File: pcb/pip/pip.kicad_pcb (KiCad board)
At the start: 2 copper layers, 41.9 x 23.9 mm, 30 parts, among them J1 USBPCB, Q1 BC847, SW1 FLASH, SW2 RESET, SW3 BUTTON_A, SW4 BUTTON_B, U1 74HC595, U2 W25Q32JVSS, U3 CH552G

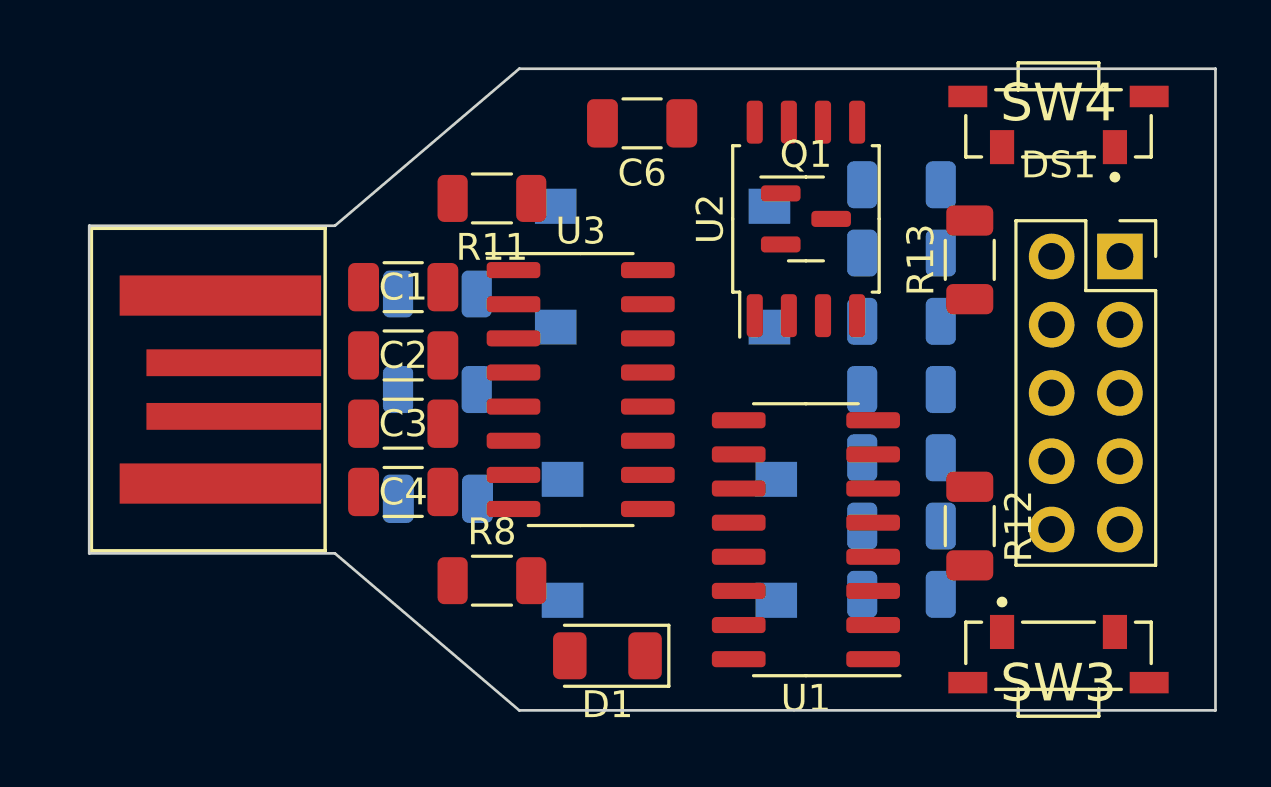
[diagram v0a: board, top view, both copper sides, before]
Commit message: pcb design
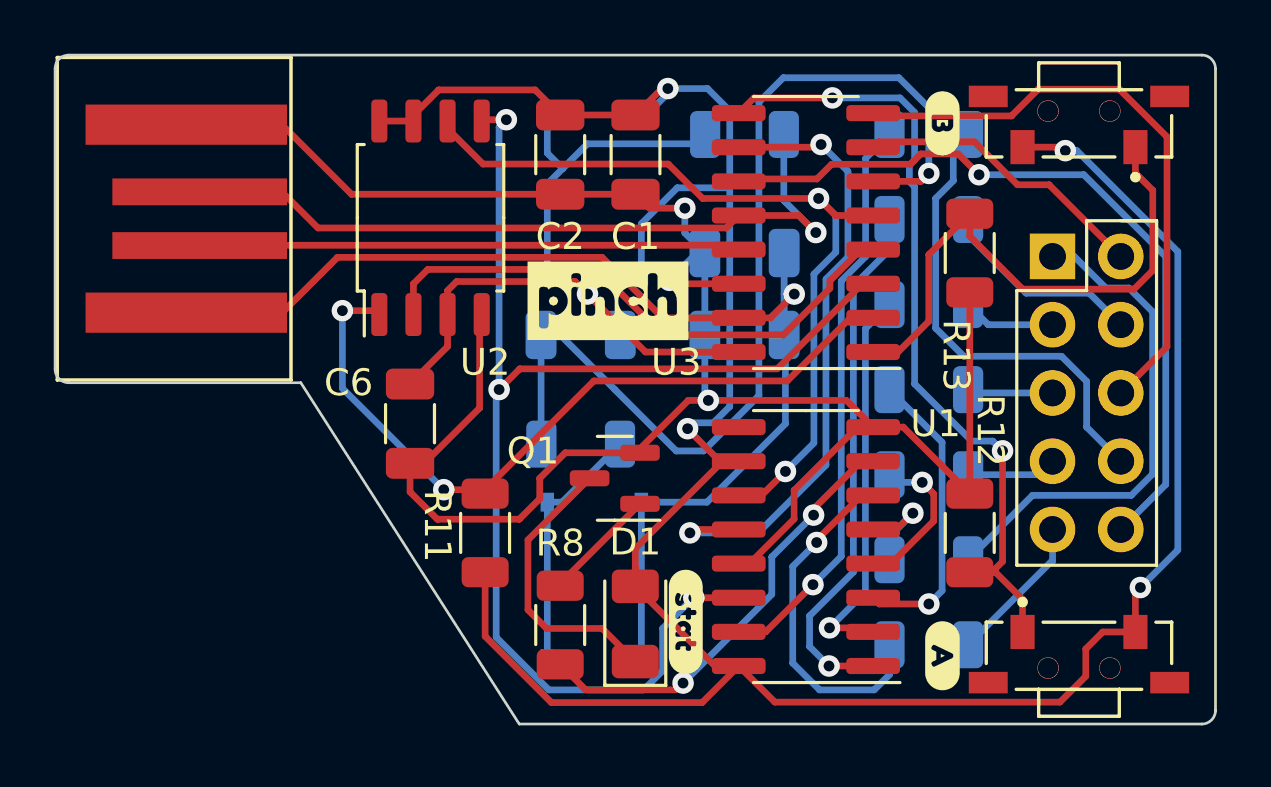
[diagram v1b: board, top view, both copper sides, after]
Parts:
- added kibuzzard-63727E71: G***, kibuzzard-63727E71, F.Cu at (149.9, 101.3)
- added kibuzzard-63727E80: G***, kibuzzard-63727E80, F.Cu at (149.9, 81.5)
- added kibuzzard-637287DB: G***, kibuzzard-637287DB, F.Cu at (137.4, 88.1)
- added kibuzzard-63728AEE: G***, kibuzzard-63728AEE, B.Cu at (133.3, 98.6)
- added kibuzzard-63728AF8: G***, kibuzzard-63728AF8, B.Cu at (133.3, 84.3)
- added kibuzzard-63728B2A: G***, kibuzzard-63728B2A, F.Cu at (140.3, 100.1)
- added kibuzzard-63728C1B: G***, kibuzzard-63728C1B, B.Cu at (143.0, 98.7)
- C3, C4: moved to B.Cu
- DS1: footprint SparkFun-Connectors:Display_2531AB -> libraries:Display_2531AB
- J1: footprint SparkFun-Connectors:USB-A-PCB -> libraries:USB-A-PCB
- SW1, SW2: footprint Button_Switch_SMD:SW_Push_1P1T_NO_6x6mm_H9.5mm -> libraries:SW_Push_45x45mm_H1.5mm
- moved C4 15.5 mm to (142.5, 86.4), turned to 180 degrees
- moved C6 14.1 mm to (130.0, 92.7), turned to 90 degrees
- moved U2 14.0 mm to (130.8, 85.0)
- moved C3 13.1 mm to (142.5, 89.4), turned to 180 degrees
- moved R9 12.9 mm to (142.5, 81.9)
- moved R11 12.4 mm to (132.8, 96.8), turned to 90 degrees
- moved Q1 12.0 mm to (137.7, 94.7), turned to 180 degrees
- moved U3 10.2 mm to (144.8, 85.6), turned to 180 degrees
- moved C1 9.95 mm to (138.4, 82.7), turned to -90 degrees
- moved C2 9.48 mm to (135.6, 82.7), turned to -90 degrees
- moved C5 8.09 mm to (136.4, 89.4), turned to 0 degrees
- moved J1 6.48 mm to (121.9, 85.1)
- moved R10 5.71 mm to (136.4, 93.5), turned to 0 degrees
- moved SW1 3.59 mm to (136.9, 84.3), turned to -90 degrees
- moved SW2 3.18 mm to (136.9, 98.6), turned to -90 degrees
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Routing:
- net VCC: track 0.00 -> 119.7 mm, vias 0 -> 5
- net GND: track 0.00 -> 83.2 mm, vias 0 -> 3
- net P1.5: track 0.00 -> 48.8 mm, vias 0 -> 3
- net VBUS: track 0.00 -> 43.9 mm, vias 0 -> 1
- net RESET: track 0.00 -> 37.5 mm, vias 0 -> 1
- net P1.7: track 0.00 -> 30.8 mm, vias 0 -> 2
- net P1.1: track 0.00 -> 30.7 mm, vias 0 -> 2
- net P3.4: track 0.00 -> 28.7 mm, vias 0 -> 1
- net P1.4: track 0.00 -> 28.4 mm, vias 0 -> 2
- net P3.6: track 0.00 -> 28.1 mm, vias 0 -> 1
- net P3.3: track 0.00 -> 23.8 mm, vias 0 -> 2
- net P3.0: track 0.00 -> 22.4 mm
- net Net-(R1-Pad1): track 0.00 -> 21.4 mm, vias 0 -> 1
- net P1.6: track 0.00 -> 21.0 mm
- net P3.2: track 0.00 -> 20.8 mm
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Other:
- board size 41.9 x 23.9 mm -> 43.2 x 24.9 mm
